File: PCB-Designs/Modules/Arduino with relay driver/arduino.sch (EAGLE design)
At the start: 40 parts, among them T1 BC547, T2 BC547, T3 BC547, T4 BC547

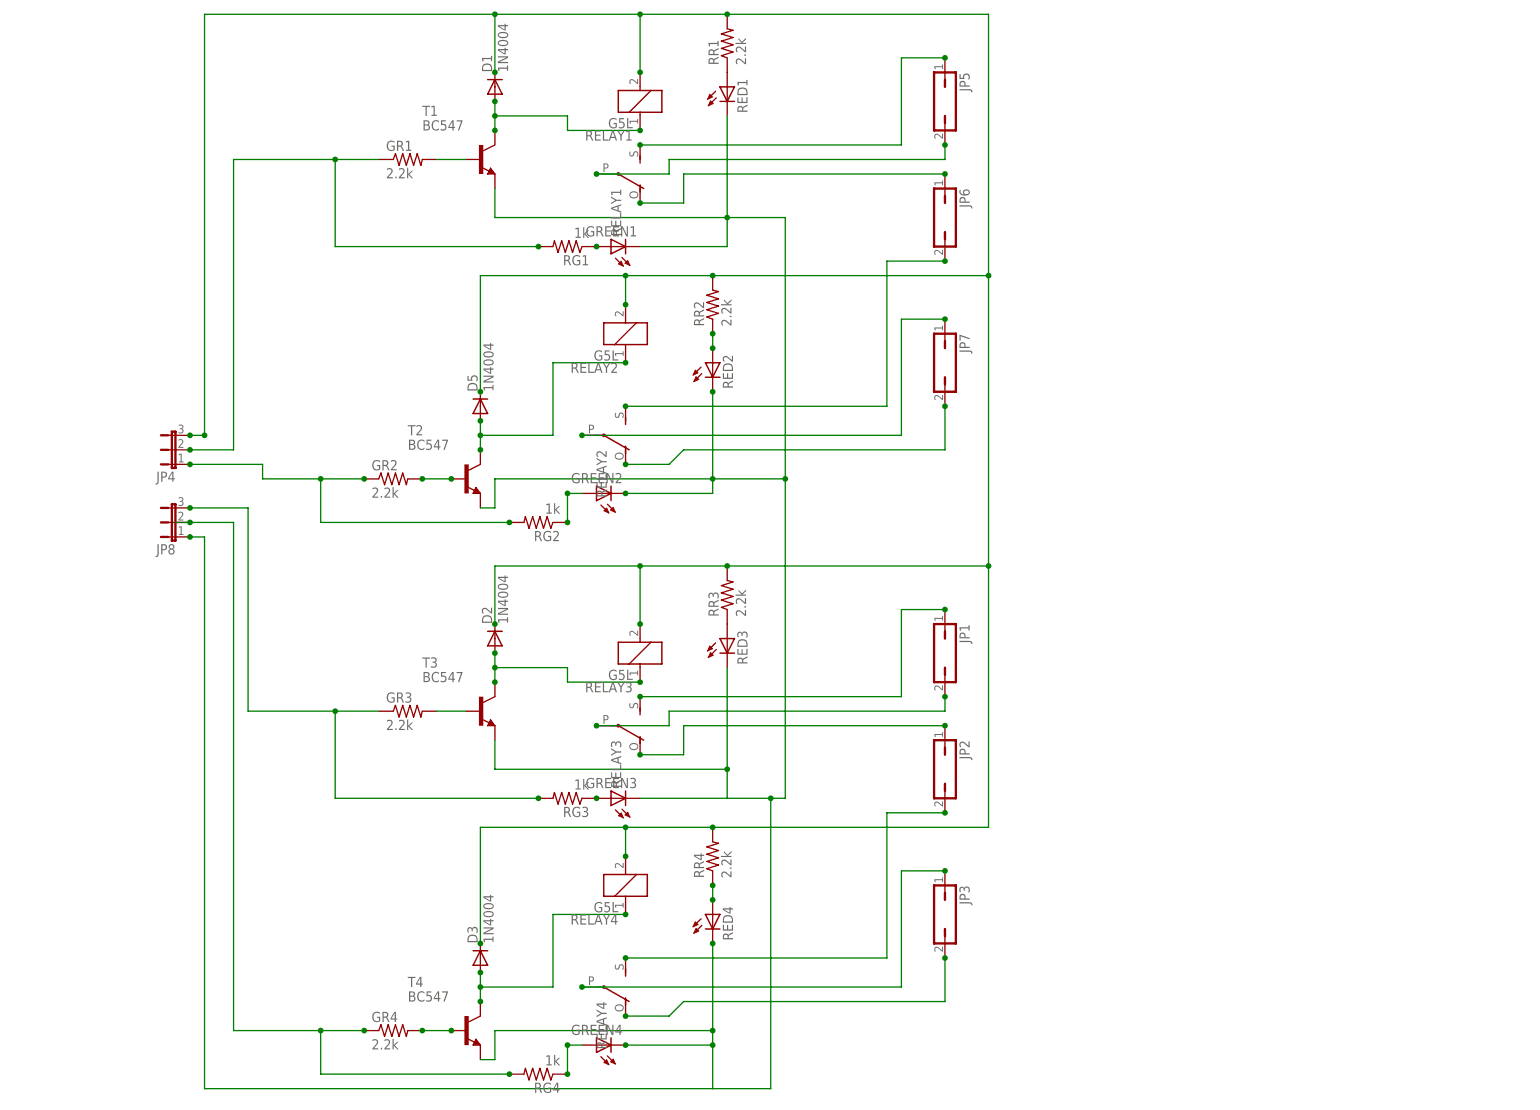
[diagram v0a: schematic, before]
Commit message: made by shankar
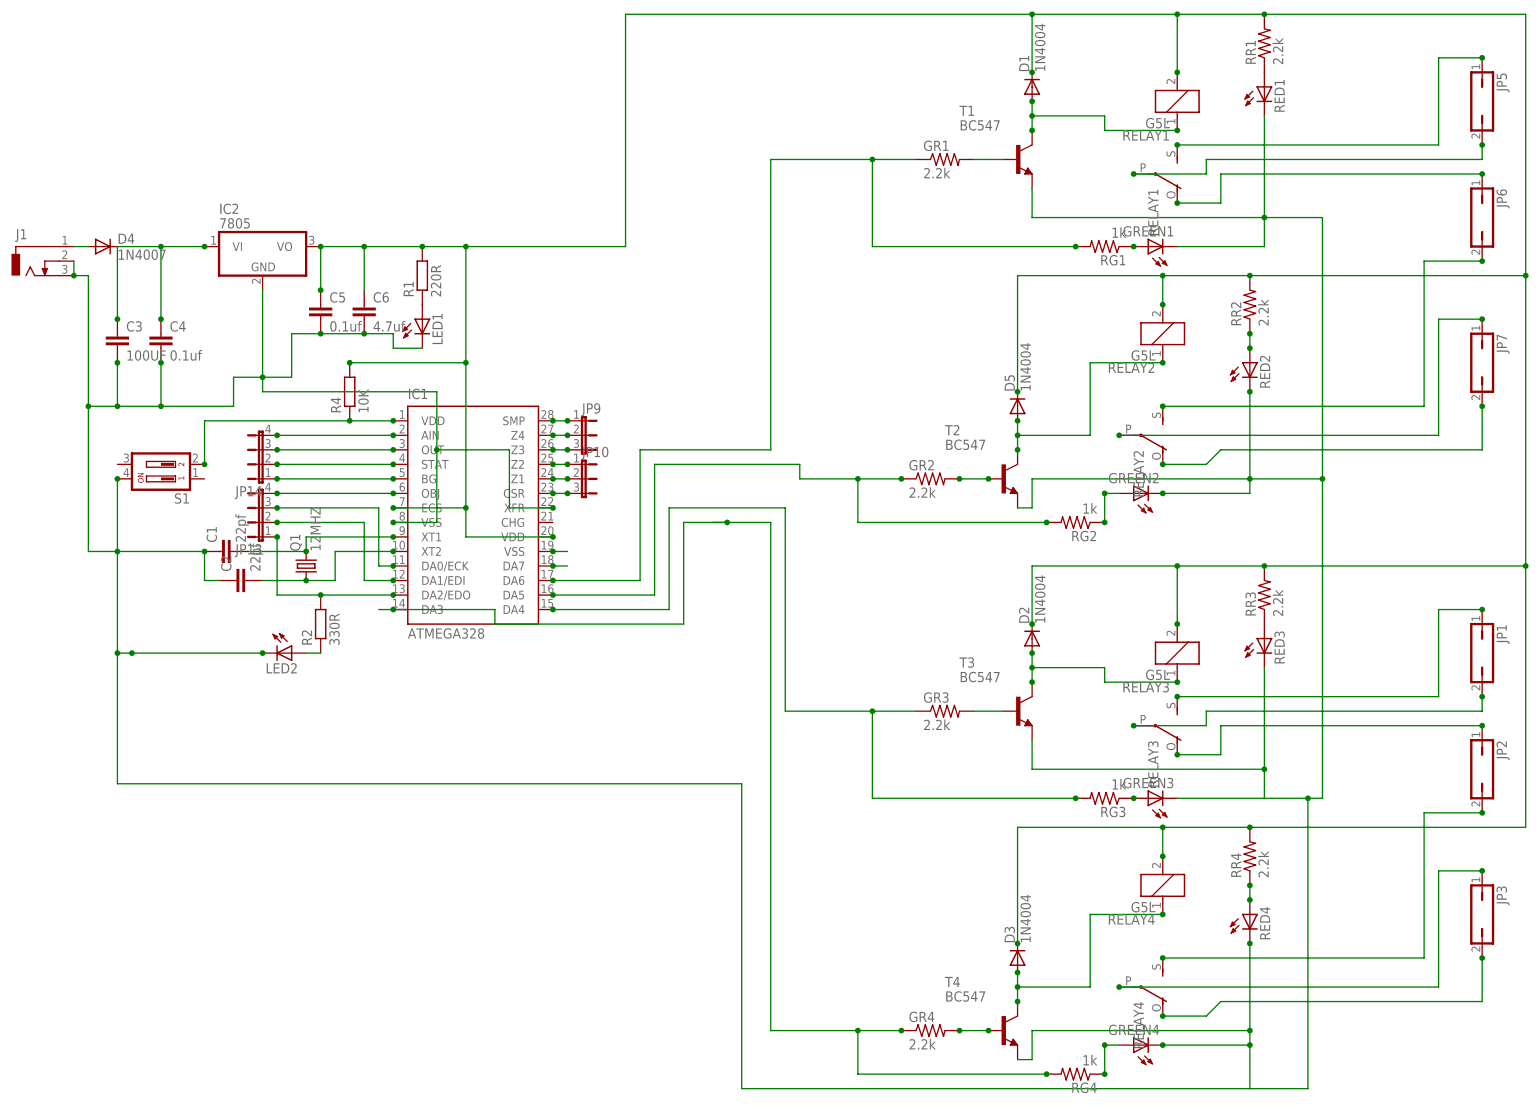
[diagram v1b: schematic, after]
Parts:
- removed JP4, JP8: (no value), jumper:JP2E
- added C1, C2: 22pf, capacitor-wima:C2.5/2
- added C3: 100UF, capacitor-wima:C2.5/2
- added C4, C5: 0.1uf, capacitor-wima:C2.5/2
- added C6: 4.7uf, capacitor-wima:C2.5/2
- added D4: 1N4007, diode:1N4004
- added IC1: ATMEGA328, quantum-research-group:QT9701BD
- added IC2: 7805, linear:786TV
- added J1: (no value), con-jack:DCJ0303
- added JP10, JP9: (no value), jumper:JP2E
- added JP13, JP14: (no value), jumper:JP4E
- added LED1, LED2: (no value), led:LED3MM
- added Q1: 12MHZ, crystal:CRYSTALHC49S
- added R1: 220R, rcl:R-EU_0207/10
- added R2: 330R, rcl:R-EU_0207/10
- added R4: 10K, rcl:R-EU_0207/10
- added S1: (no value), switch-dil:DP02
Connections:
- removed net N$16: GR2.1, JP4.1, RG2.2
- removed net N$2: D1.C, D2.C, D3.C, D5.C, JP4.3, RELAY11.2, RELAY21.2, RELAY31.2, RELAY41.2, RR1.2, RR2.2, RR3.2, RR4.2
- removed net N$23: GREEN1.C, GREEN2.C, GREEN3.C, GREEN4.C, JP8.1, RED1.C, RED2.C, RED3.C, RED4.C, T1.E, T2.E, T3.E, T4.E
- removed net N$25: GR3.1, JP8.3, RG3.2
- removed net N$34: GR4.1, JP8.2, RG4.2
- removed net N$6: GR1.1, JP4.2, RG1.2
- new net N$14: C2.2, IC1.XT2, Q1.1
- new net N$21: C1.1, C2.1, C3.2, C4.2, C5.2, C6.2, GREEN1.C, GREEN2.C, GREEN3.C, GREEN4.C, IC1.VSS, IC1.XFR, IC2.GND, J1.2, J1.3, LED1.C, LED2.C, RED1.C, RED2.C, RED3.C, RED4.C, S1.4, T1.E, T2.E, T3.E, T4.E
- new net N$32: C3.1, C4.1, D4.C, IC2.VI
- new net N$39: D4.A, J1.1
- new net N$4: C1.2, IC1.XT1, Q1.2
- new net N$40: C5.1, C6.1, D1.C, D2.C, D3.C, D5.C, IC1.ECS, IC1.VDD@1, IC2.VO, R1.2, R4.2, RELAY11.2, RELAY21.2, RELAY31.2, RELAY41.2, RR1.2, RR2.2, RR3.2, RR4.2
- new net N$41: LED1.A, R1.1
- new net N$42: IC1.SMP, JP9.1
- new net N$43: IC1.Z4, JP9.2
- new net N$44: IC1.Z3, JP9.3
- new net N$45: IC1.Z2, JP10.1
- new net N$46: IC1.Z1, JP10.2
- new net N$47: IC1.CSR, JP10.3
- new net N$48: IC1.AIN, JP14.4
- new net N$49: IC1.OUT, JP14.3
- new net N$50: IC1.STAT, JP14.2
- new net N$51: IC1.BG, JP14.1
- new net N$52: IC1.OBJ, JP13.4
- new net N$53: IC1.DA1/EDI, JP13.2
- new net N$54: IC1.DA0/ECK, JP13.3
- new net N$55: IC1.DA2/EDO, JP13.1, R2.2
- new net N$56: GR4.1, IC1.DA3, RG4.2
- new net N$57: GR3.1, IC1.DA4, RG3.2
- new net N$58: GR2.1, IC1.DA5, RG2.2
- new net N$59: GR1.1, IC1.DA6, RG1.2
- new net N$60: IC1.DA7
- new net N$61: IC1.VSS@1
- new net N$62: IC1.VDD, R4.1, S1.2
- new net N$63: LED2.A, R2.1
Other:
- moved on the sheet: D1, D2, D3, D5, GR1, GR2, GR3, GR4, GREEN1, GREEN2, GREEN3, GREEN4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
